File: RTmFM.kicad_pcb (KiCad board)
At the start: 2 copper layers, 122 x 157 mm, 58 parts, among them J1 Conn_02x04_Odd_Even, J2 Conn_01x04, J3 Conn_02x17_Odd_Even, J4 Conn_02x10_Odd_Even, J5 Micro_SD_Card, J6 Conn_01x02, J7 Conn_01x02, U1 SN75176AP, U10 74LS06, U2 SN75176AP, U7 74HCT244, U8 Pico, U9 74HCT04

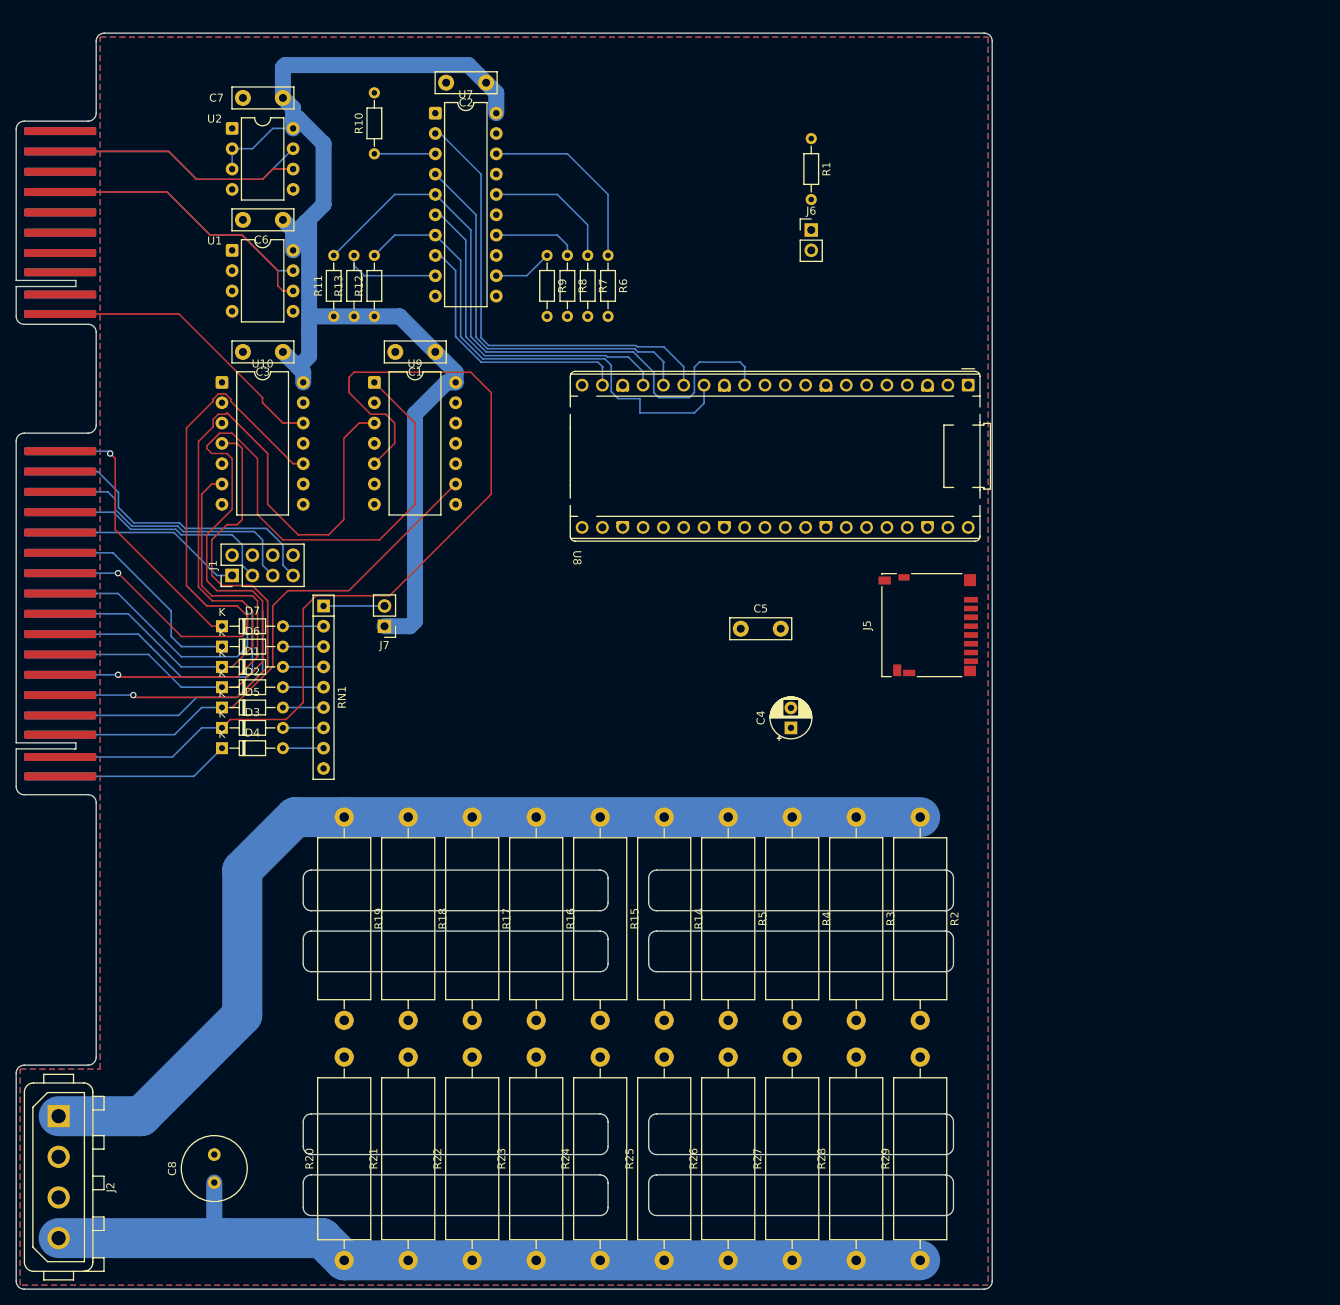
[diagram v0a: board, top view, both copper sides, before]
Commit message: Almost finished HW design
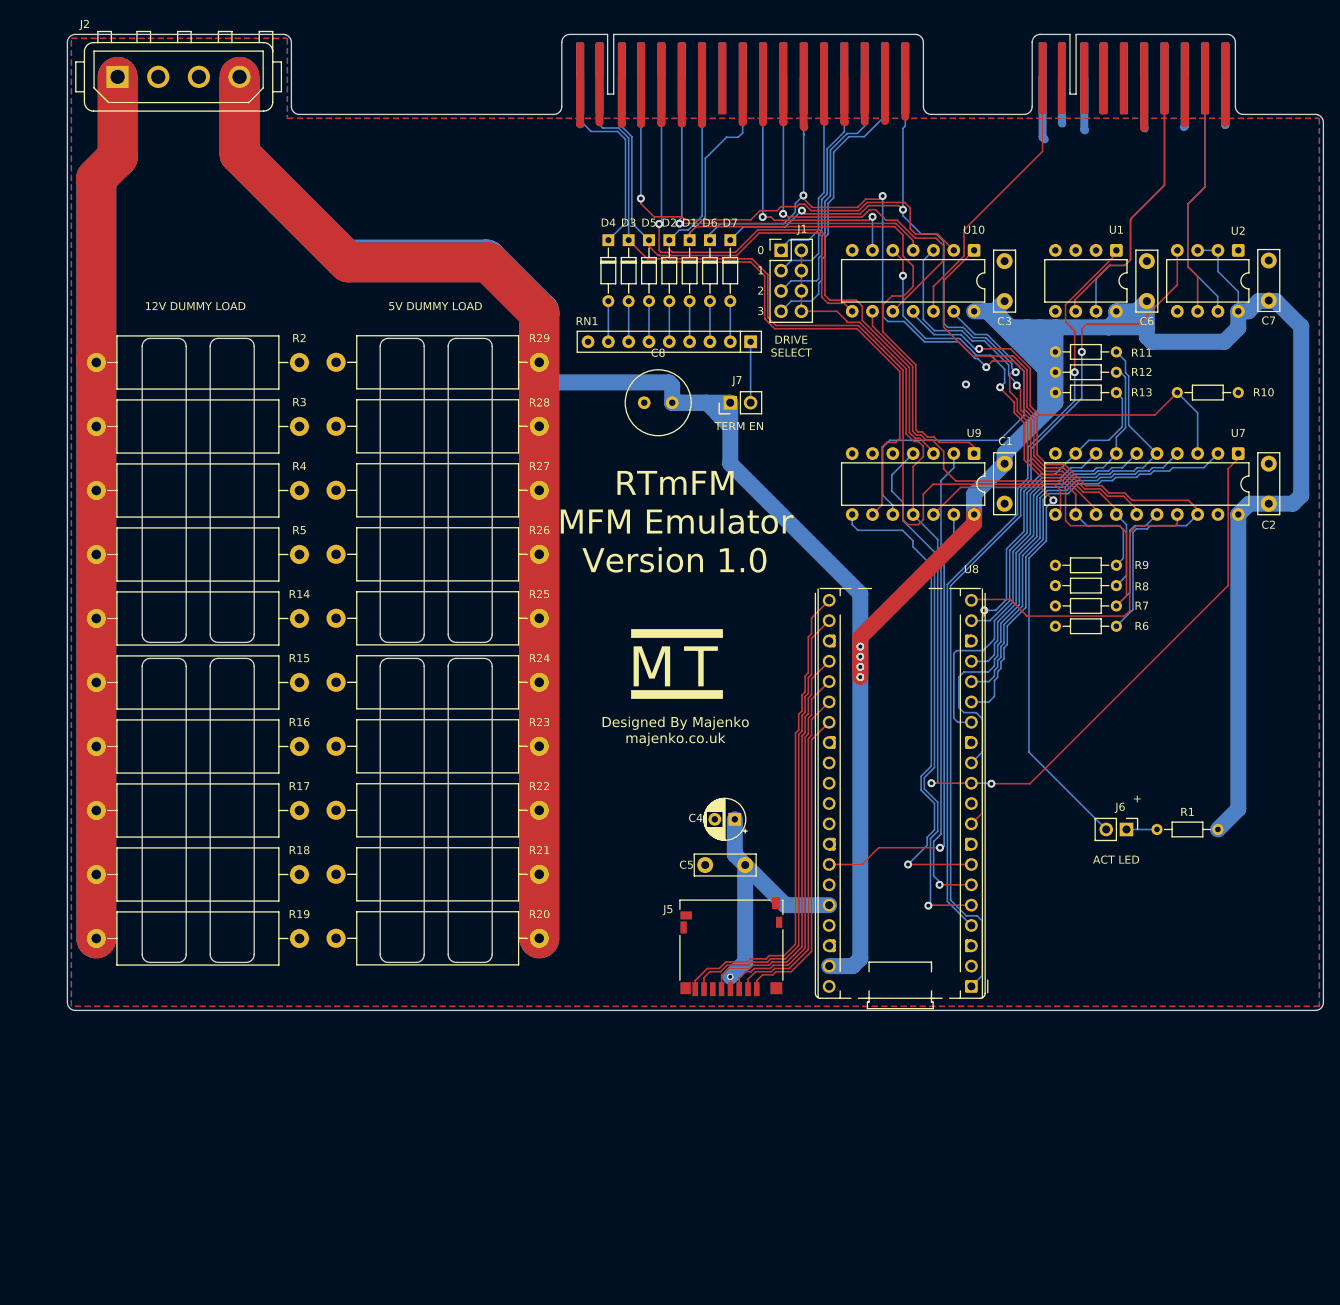
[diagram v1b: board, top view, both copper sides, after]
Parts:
- U10, U9: footprint Package_DIP:DIP-14_W10.16mm -> Package_DIP:DIP-14_W7.62mm
- moved J4 143.4 mm to (173.4, 40.2), turned to -90 degrees
- moved J2 130.1 mm to (32.7, 35.5), turned to 0 degrees
- moved U2 126.7 mm to (172.8, 57.2), turned to -90 degrees
- moved C7 125.8 mm to (176.6, 63.4), turned to 90 degrees
- moved R29 121.9 mm to (85.4, 71.1), turned to 180 degrees
- moved R2 117.6 mm to (30.0, 71.2), turned to 0 degrees
- moved C8 113.0 mm to (102.0, 76.2), turned to 180 degrees
- moved R28 111.5 mm to (85.4, 79.1), turned to 180 degrees
- moved J3 111.4 mm to (134.4, 40.2), turned to -90 degrees
- moved C2 111.1 mm to (176.6, 88.8), turned to 90 degrees
- moved U1 110.5 mm to (157.5, 57.2), turned to -90 degrees
- moved U7 109.0 mm to (172.8, 82.5), turned to -90 degrees
- moved C6 108.5 mm to (161.3, 63.5), turned to 90 degrees
- moved R3 106.8 mm to (30.0, 79.2), turned to 0 degrees
- moved R10 104.7 mm to (165.1, 74.9), turned to 0 degrees
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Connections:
- U10 pad 3: /TRACK0 -> /WRITE_FAULT
- U10 pad 4: /ocTRACK0 -> /ocWRITE_FAULT
- U10 pad 5: /WRITE_FAULT -> /INDEX
- U10 pad 6: /ocWRITE_FAULT -> /ocINDEX
- U10 pad 8: /ocINDEX -> /ocTRACK0
- U10 pad 9: /INDEX -> /TRACK0
- U8 pad 39: unconnected-(U8-VSYS-Pad39) -> VCC
- U9 pad 1: /HEAD0 -> /HEAD1
- U9 pad 2: /HSEL0 -> /HSEL1
- U9 pad 3: /HEAD1 -> /HEAD0
- U9 pad 4: /HSEL1 -> /HSEL0
- U9 pad 5: /HEAD2 -> (no net)
- U9 pad 6: /HSEL2 -> (no net)
- U9 pad 8: /RDENA -> /HSEL2
- U9 pad 9: /WRGATE -> /HEAD2
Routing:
- net VCC: track 271.4 -> 620.0 mm, vias 0 -> 4
- net GND: track 0.00 -> 144.0 mm, vias 0 -> 1
- net /DSEL: track 0.00 -> 143.9 mm, vias 0 -> 2
- net /DOUT: track 0.00 -> 110.5 mm, vias 0 -> 1
- net /WDATA: track 0.00 -> 95.3 mm, vias 0 -> 1
- net +12V: track 133.8 -> 217.6 mm
- net /STEP: track 30.4 -> 105.1 mm, vias 0 -> 3
- net /HSEL0: track 0.00 -> 66.9 mm, vias 0 -> 1
- net Net-(J6-Pin_2): track 0.00 -> 63.5 mm, vias 0 -> 1
- net /HSEL2: track 0.00 -> 61.6 mm, vias 0 -> 1
- net /SD_DAT1: track 0.00 -> 60.2 mm
- net /TRACK0: track 16.8 -> 76.8 mm
- net /DIRECTION: track 34.5 -> 93.9 mm, vias 1 -> 3
- net /HSEL1: track 0.00 -> 59.2 mm, vias 0 -> 1
- net /DRV_LED: track 0.00 -> 57.5 mm, vias 0 -> 1
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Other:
- board size 122 x 157 mm -> 157 x 122 mm
- board text added: "+"
- board text added: "0"
- board text added: "1"
- board text added: "12V DUMMY LOAD"
- board text added: "2"
- board text added: "3"
- board text added: "5V DUMMY LOAD"
- board text added: "ACT LED"
- board text added: "DRIVE SELECT"
- board text added: "Designed By Majenko"
- board text added: "M"
- board text added: "RTmFM MFM Emulator Version 1.0"
- board text added: "T"
- board text added: "TERM EN"
- board text added: "majenko.co.uk"
